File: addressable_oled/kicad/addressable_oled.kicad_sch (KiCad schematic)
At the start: 6 parts, among them J1 Conn_01x06_Pin, J2 Conn_01x03_Socket, U1 SLG46826G

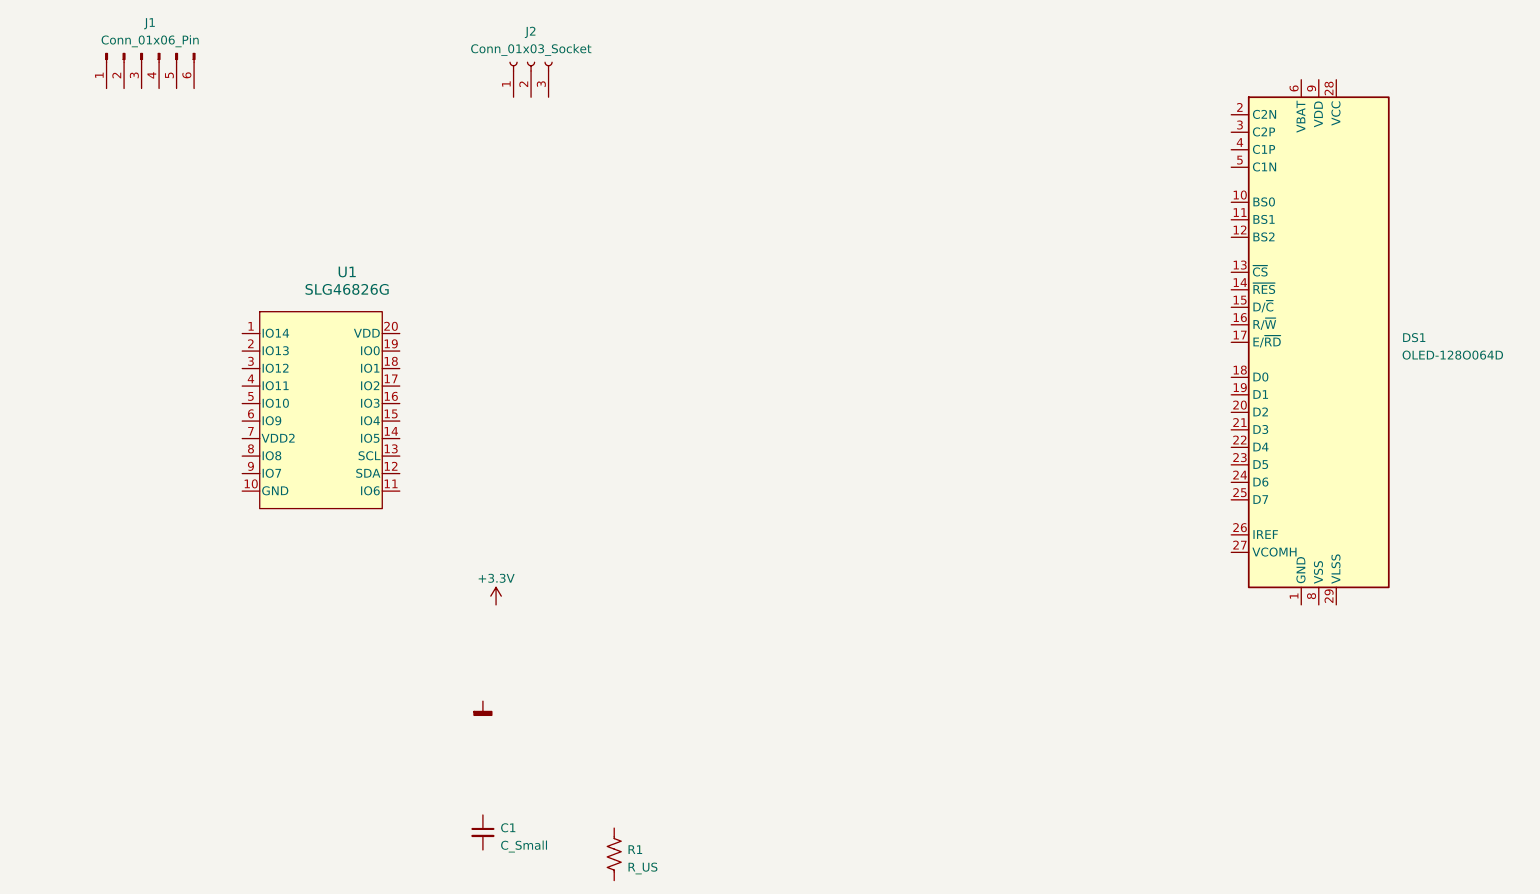
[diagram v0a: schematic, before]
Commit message: Work in progress. First pass of the schematic.
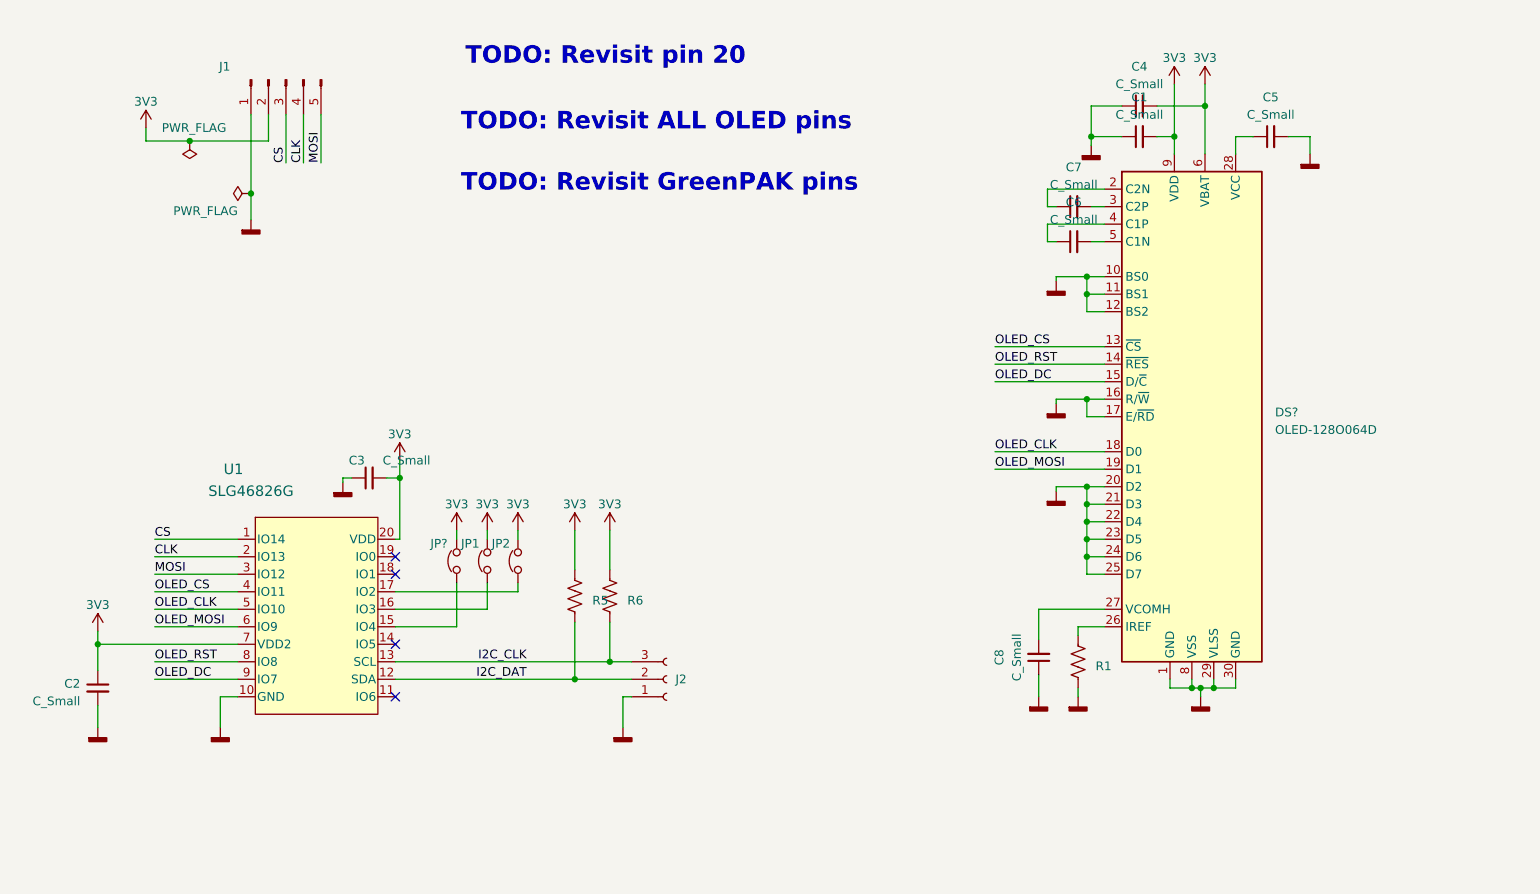
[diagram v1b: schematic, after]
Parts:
- added C2, C3, C4, C5, C6, C7, C8: C_Small, symbol Device:C_Small
- added JP1, JP2, JP?: Jumper_2_Open, symbol addressable_oled:Jumper_2_Open
- added R5, R6: R_US, symbol Device:R_US
- J1: value Conn_01x06_Pin -> Conn_01x05_Pin; symbol Connector:Conn_01x06_Pin -> Connector:Conn_01x05_Pin
- renumbered DS1 to DS?
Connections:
- net GND: now also C1.1, DS?.1 (GND), DS?.10 (BS0), DS?.11 (BS1), DS?.12 (BS2), DS?.16 (R/~{W}), DS?.17 (E/~{RD}), DS?.20 (D2), DS?.21 (D3), DS?.22 (D4), DS?.23 (D5), DS?.24 (D6), DS?.25 (D7), DS?.29 (VLSS), DS?.30 (GND), DS?.8 (VSS), J1.1 (Pin_1), J2.1 (Pin_1), R1.2, U1.10 (GND), C2.2, C3.1, C4.1, C5.2, C8.1
- net 3V3: now reaches J1.2 (Pin_2)
- net 3V3: now also C1.2, DS?.6 (VBAT), DS?.9 (VDD), U1.20 (VDD), U1.7 (VDD2), C2.1, C3.2, C4.2, JP1.2, JP2.2, JP?.2, R5.1, R6.1
- net CS: now reaches J1.3 (Pin_3)
- net CS: now also U1.1 (IO14)
- net CLK: now reaches J1.4 (Pin_4)
- net CLK: now also U1.2 (IO13)
- net MOSI: now reaches J1.5 (Pin_5)
- net MOSI: now also U1.3 (IO12)
- net at R1.1: now also DS?.26 (IREF)
- net OLED_CS: now reaches DS?.13 (~{CS})
- net OLED_CS: now also U1.4 (IO11)
- net OLED_RST: now reaches DS?.14 (~{RES})
- net OLED_RST: now also U1.8 (IO8)
- net OLED_DC: now reaches DS?.15 (D/~{C})
- net OLED_DC: now also U1.9 (IO7)
- net OLED_CLK: now reaches DS?.18 (D0)
- net OLED_CLK: now also U1.5 (IO10)
- net OLED_MOSI: now reaches DS?.19 (D1)
- net OLED_MOSI: now also U1.6 (IO9)
- net at DS?.2 (C2N): now also C7.1
- net at DS?.27 (VCOMH): now also C8.2
- net at DS?.28 (VCC): now also C5.1
- net at DS?.3 (C2P): now also C7.2
- net at DS?.4 (C1P): now also C6.1
- net at DS?.5 (C1N): now also C6.2
- net I2C_DAT: now reaches J2.2 (Pin_2)
- net I2C_DAT: now also U1.12 (SDA), R5.2
- net I2C_CLK: now reaches J2.3 (Pin_3)
- net I2C_CLK: now also U1.13 (SCL), R6.2
- net at U1.15 (IO4): now also JP?.1~ (A)
- net at U1.16 (IO3): now also JP1.1~ (A)
- net at U1.17 (IO2): now also JP2.1~ (A)
- no-connect marks 0 -> 4
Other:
- note added: "TODO: Revisit ALL OLED pins"
- note added: "TODO: Revisit GreenPAK pins"
- note added: "TODO: Revisit pin 20"
- moved on the sheet: C1, J2, U1
